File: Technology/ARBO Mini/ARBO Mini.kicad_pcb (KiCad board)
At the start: 4 copper layers, 35.6 x 15.2 mm, 86 parts, among them J1 USB_B_Micro, J2 Micro_SD_Card_473093351, J3 Conn_01x10, SW1 SW_SPST, U1 MCP73831-2-OT, U2 MAX828, U3 ICM-20948, U4 SPX3819M5-L-3-3, U5 MAX1726EUK18+, U6 ATSAMD21G18A-AUT, U7 ADS1294, U8 SN74AUP1G98, U9 MB85RSxM_WLP8, Y1 Crystal

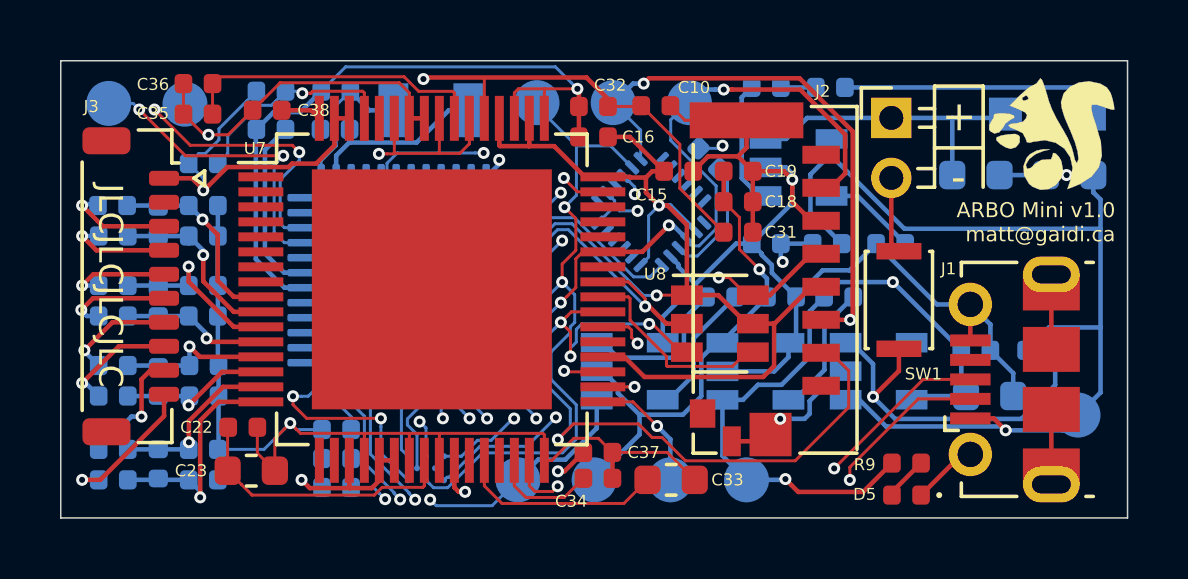
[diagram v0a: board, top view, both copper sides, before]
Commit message: ARBO mini sent to JSTPCB for fab
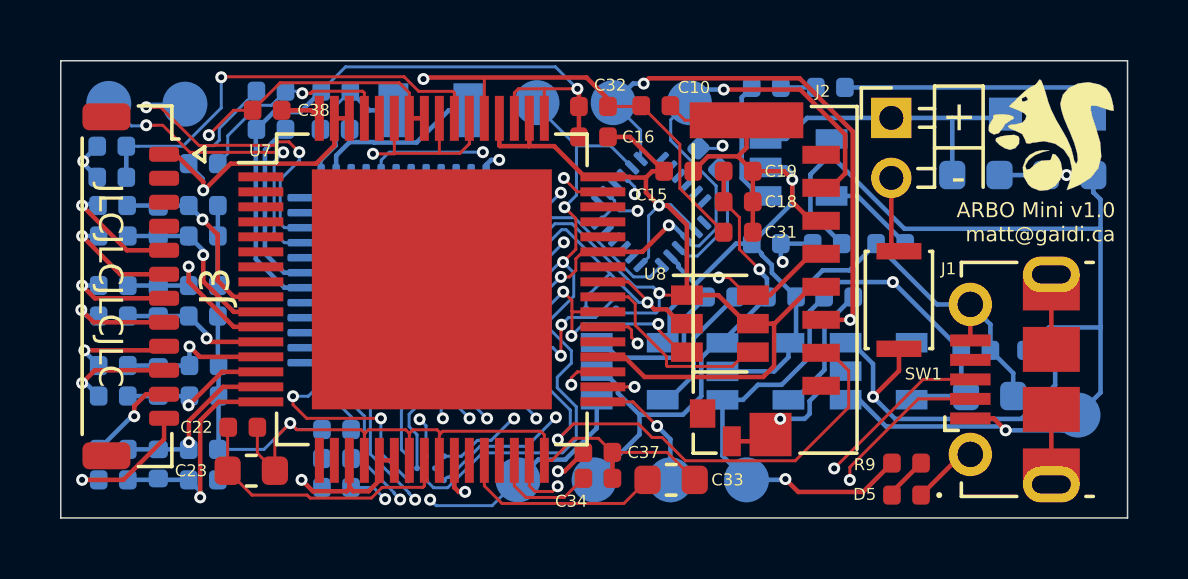
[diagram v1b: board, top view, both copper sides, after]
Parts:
- added U10: SiT1532, ARBO:SiT1532, B.Cu at (123.4, 61.4)
- C35, C36: moved to B.Cu
- J3: footprint Connector_Hirose:Hirose_DF52-10S-0.8H_1x10-1MP_P0.80mm_Horizontal -> Connector_Hirose:Hirose_DF52-12S-0.8H_1x12-1MP_P0.80mm_Horizontal
- moved C36 4.24 mm to (107.1, 57.2)
- moved C35 3.07 mm to (107.1, 56.2)
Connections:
- J3 pad 10: HI_IN1P -> HI_IN2P
- J3 pad 3: HI_IN4N -> (no net)
- J3 pad 4: HI_IN4P -> (no net)
- J3 pad 5: HI_IN3N -> HI_IN4N
- J3 pad 6: HI_IN3P -> HI_IN4P
- J3 pad 7: HI_IN2N -> HI_IN3N
- J3 pad 8: HI_IN2P -> HI_IN3P
- J3 pad 9: HI_IN1N -> HI_IN2N
- U6 pad 23: SD_CS -> Net-(U10-Pad2)
- U6 pad 24: EC_START -> SD_CS
- U6 pad 25: (no net) -> EC_START
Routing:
- net Net-(U10-Pad2): track 0.00 -> 5.16 mm, vias 0 -> 2
- net Net-(C35-Pad1): track 10.2 -> 14.6 mm, vias 0 -> 1
- net +3V3: track 92.6 -> 94.6 mm
- net GNDD: track 120.6 -> 122.2 mm
- net HI_BIAS: track 12.5 -> 13.4 mm
- net HI_IN1N: track 4.00 -> 3.14 mm
- net SCK: track 33.5 -> 34.2 mm
- net Net-(TP11-Pad1): track 9.88 -> 10.5 mm
- net MISO: track 30.9 -> 31.5 mm
- net SD_CS: track 18.4 -> 17.8 mm
- net -1V8: track 79.6 -> 79.2 mm, vias 4 -> 5
